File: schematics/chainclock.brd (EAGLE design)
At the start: 72.7 x 40 mm, 19 parts, among them SW1 ROTARTY_ENCODER

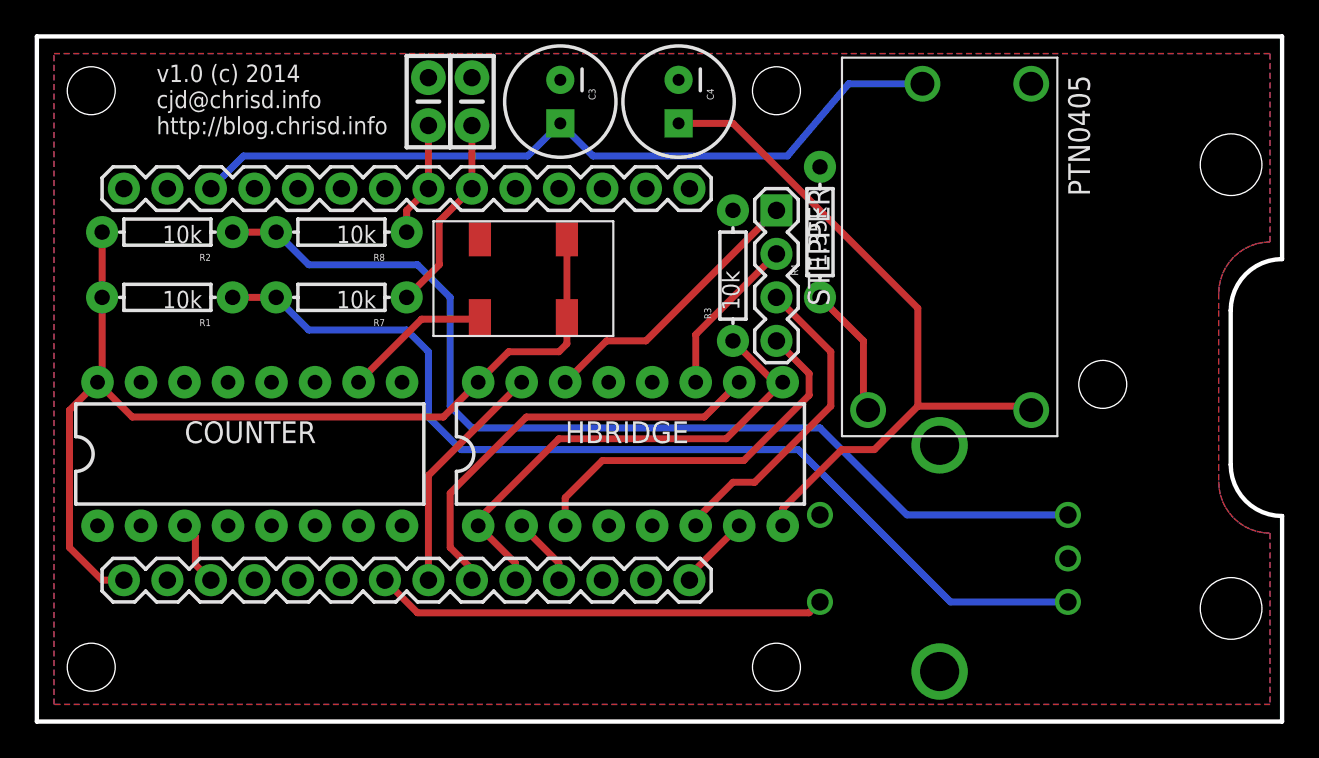
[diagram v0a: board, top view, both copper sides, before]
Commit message: New board layout
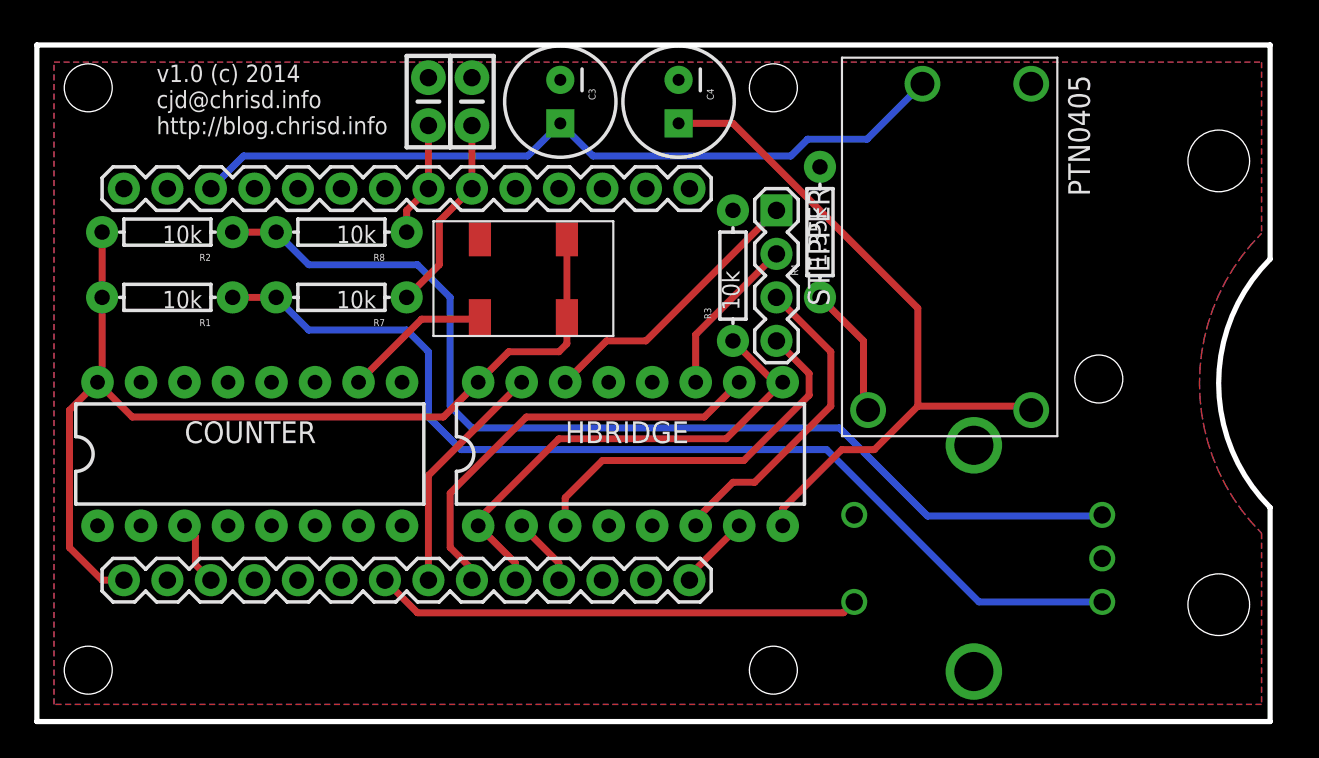
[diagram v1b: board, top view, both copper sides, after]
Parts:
- moved U$2 25.8 mm to (81.8, 19.9)
- moved SW1 2.00 mm to (54.7, 9.53)
- moved U$3 1.00 mm to (66.9, 29.8)
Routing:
- net N$5: track 59.3 -> 61.4 mm
- net N$2: track 58.4 -> 60.4 mm
- net RENBTN: track 26.5 -> 28.5 mm
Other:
- board size 72.7 x 40 mm -> 72 x 39.5 mm
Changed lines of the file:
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@@
 <setting verticaltext="up"/>
 </settings>
-<grid distance="0.025" unitdist="inch" unit="inch" style="lines" multiple="1" display="yes" altdistance="0.025" altunitdist="inch" altunit="inch"/>
+<grid distance="0.5" unitdist="mm" unit="mm" style="lines" multiple="1" display="yes" altdistance="0.025" altunitdist="inch" altunit="inch"/>
 <layers>
 <layer number="1" name="Top" color="4" fill="1" visible="yes" active="yes"/>
@@
 <board>
 <plain>
-<hole x="3.175" y="3.175" drill="2.8"/>
-<hole x="3.175" y="36.83" drill="2.8"/>
-<wire x1="0" y1="0" x2="0" y2="40" width="0.254" layer="20"/>
-<wire x1="0" y1="40" x2="72.7" y2="40" width="0.254" layer="20"/>
-<wire x1="72.7" y1="0" x2="0" y2="0" width="0.254" layer="20"/>
-<hole x="62.23" y="19.685" drill="2.8"/>
-<wire x1="72.7" y1="0" x2="72.7" y2="12" width="0.254" layer="20"/>
-<wire x1="72.7" y1="12" x2="69.7" y2="15" width="0.254" layer="20" curve="-90"/>
-<wire x1="69.7" y1="15" x2="69.7" y2="24" width="0.254" layer="20"/>
-<wire x1="69.7" y1="24" x2="72.7" y2="27" width="0.254" layer="20" curve="-90"/>
-<wire x1="72.7" y1="27" x2="72.7" y2="40" width="0.254" layer="20"/>
+<hole x="3" y="3" drill="2.8"/>
+<hole x="3" y="37" drill="2.8"/>
+<hole x="62" y="20" drill="2.8"/>
 <text x="6.985" y="34.29" size="1.016" layer="21">v1.0 (c) 2014
 cjd@chrisd.info
 http://blog.chrisd.info</text>
-<hole x="43.18" y="3.175" drill="2.8"/>
-<hole x="43.18" y="36.83" drill="2.8"/>
+<hole x="43" y="3" drill="2.8"/>
+<hole x="43" y="37" drill="2.8"/>
+<wire x1="0" y1="0" x2="0" y2="39.5" width="0.3048" layer="20"/>
+<wire x1="0" y1="39.5" x2="72" y2="39.5" width="0.3048" layer="20"/>
+<wire x1="72" y1="39.5" x2="72" y2="27" width="0.3048" layer="20"/>
+<wire x1="72" y1="27" x2="72" y2="12.5" width="0.3048" layer="20" curve="90"/>
+<wire x1="72" y1="12.5" x2="72" y2="0" width="0.3048" layer="20"/>
+<wire x1="0" y1="0" x2="72" y2="0" width="0.3048" layer="20"/>
 </plain>
 <attributes>
@@
 <element name="C4" library="SparkFun-Passives" package="CPOL-RADIAL-100UF-25V" value="" x="37.465" y="36.195" rot="R270"/>
 <element name="R4" library="SparkFun-Resistors" package="AXIAL-0.3EZ" value="1.35k" x="45.72" y="28.575" rot="R90"/>
-<element name="U$2" library="desjardins" package="NEMA14" value="" x="100.33" y="1.905" rot="R90"/>
-<element name="U$3" library="desjardins" package="LOGO" value="" x="67.945" y="29.845" rot="MR270"/>
-<element name="SW1" library="SparkFun-Electromechanical" package="ROTARY_ENC_PLAIN" value="ROTARTY_ENCODER" x="52.705" y="9.525" rot="MR180"/>
+<element name="U$2" library="desjardins" package="NEMA14" value="" x="81.83" y="19.905" rot="R90"/>
+<element name="U$3" library="desjardins" package="LOGO" value="" x="66.945" y="29.845" rot="MR270"/>
+<element name="SW1" library="SparkFun-Electromechanical" package="ROTARY_ENC_PLAIN" value="ROTARTY_ENCODER" x="54.705" y="9.525" rot="MR180"/>
 <element name="C5" library="SparkFun-Capacitors" package="CAP-PTH-SMALL-KIT" value=".01uf" x="22.86" y="36.195" rot="R90"/>
 <element name="C6" library="SparkFun-Capacitors" package="CAP-PTH-SMALL-KIT" value=".01uf" x="25.4" y="36.195" rot="R90"/>
@@
 <polygon width="0.4064" layer="16">
 <vertex x="1" y="1"/>
-<vertex x="1" y="39"/>
-<vertex x="72" y="39"/>
-<vertex x="72" y="28" curve="90"/>
-<vertex x="69" y="25"/>
-<vertex x="69" y="24"/>
-<vertex x="69" y="15"/>
-<vertex x="69" y="14" curve="90"/>
-<vertex x="72" y="11"/>
-<vertex x="72" y="1"/>
+<vertex x="1" y="38.5"/>
+<vertex x="71.5" y="38.5"/>
+<vertex x="71.5" y="28.5" curve="90"/>
+<vertex x="71.5" y="11"/>
+<vertex x="71.5" y="1"/>
 </polygon>
 <polygon width="0.4064" layer="1">
 <vertex x="1" y="1"/>
-<vertex x="1" y="39"/>
-<vertex x="72" y="39"/>
-<vertex x="72" y="28" curve="90"/>
-<vertex x="69" y="25"/>
-<vertex x="69" y="24"/>
-<vertex x="69" y="15"/>
-<vertex x="69" y="14" curve="90"/>
-<vertex x="72" y="11"/>
-<vertex x="72" y="1"/>
+<vertex x="1" y="38.5"/>
+<vertex x="71.5" y="38.5"/>
+<vertex x="71.5" y="28.5" curve="90"/>
+<vertex x="71.5" y="11"/>
+<vertex x="71.5" y="1"/>
 </polygon>
 </signal>
@@
 <wire x1="10.16" y1="31.115" x2="12.065" y2="33.02" width="0.4064" layer="16"/>
 <wire x1="12.065" y1="33.02" x2="28.655" y2="33.02" width="0.4064" layer="16"/>
-<wire x1="51.704" y1="37.236" x2="47.396" y2="37.236" width="0.4064" layer="16"/>
-<wire x1="47.396" y1="37.236" x2="43.815" y2="33.02" width="0.4064" layer="16"/>
 <wire x1="28.655" y1="33.02" x2="30.56" y2="34.925" width="0.4064" layer="16"/>
-<wire x1="43.815" y1="33.02" x2="32.465" y2="33.02" width="0.4064" layer="16"/>
+<wire x1="44.02" y1="33.02" x2="32.465" y2="33.02" width="0.4064" layer="16"/>
 <wire x1="32.465" y1="33.02" x2="30.56" y2="34.925" width="0.4064" layer="16"/>
+<wire x1="44.02" y1="33.02" x2="45" y2="34" width="0.4064" layer="16"/>
+<wire x1="45" y1="34" x2="48.468" y2="34" width="0.4064" layer="16"/>
+<wire x1="48.468" y1="34" x2="51.704" y2="37.236" width="0.4064" layer="16"/>
 </signal>
 <signal name="3V32">
@@
 <wire x1="15.875" y1="22.86" x2="21.59" y2="22.86" width="0.4064" layer="16"/>
 <wire x1="22.86" y1="17.78" x2="24.765" y2="15.875" width="0.4064" layer="16"/>
-<wire x1="24.765" y1="15.875" x2="44.45" y2="15.875" width="0.4064" layer="16"/>
-<wire x1="44.45" y1="15.875" x2="53.34" y2="6.985" width="0.4064" layer="16"/>
-<wire x1="53.34" y1="6.985" x2="60.198" y2="6.985" width="0.4064" layer="16"/>
+<wire x1="24.765" y1="15.875" x2="46.11" y2="15.875" width="0.4064" layer="16"/>
+<wire x1="55" y1="6.985" x2="62.198" y2="6.985" width="0.4064" layer="16"/>
 <wire x1="22.86" y1="17.78" x2="22.86" y2="21.59" width="0.4064" layer="16"/>
 <wire x1="22.86" y1="21.59" x2="21.59" y2="22.86" width="0.4064" layer="16"/>
+<wire x1="46.11" y1="15.875" x2="55" y2="6.985" width="0.4064" layer="16"/>
 </signal>
 <signal name="N$5">
@@
 <wire x1="24.13" y1="24.765" x2="24.13" y2="18.415" width="0.4064" layer="16"/>
 <wire x1="24.13" y1="18.415" x2="25.4" y2="17.145" width="0.4064" layer="16"/>
-<wire x1="25.4" y1="17.145" x2="45.72" y2="17.145" width="0.4064" layer="16"/>
-<wire x1="45.72" y1="17.145" x2="50.8" y2="12.065" width="0.4064" layer="16"/>
-<wire x1="50.8" y1="12.065" x2="60.198" y2="12.065" width="0.4064" layer="16"/>
+<wire x1="25.4" y1="17.145" x2="46.855" y2="17.145" width="0.4064" layer="16"/>
+<wire x1="46.855" y1="17.145" x2="52" y2="12" width="0.4064" layer="16"/>
+<wire x1="52" y1="12" x2="62.133" y2="12" width="0.4064" layer="16"/>
+<wire x1="62.133" y1="12" x2="62.198" y2="12.065" width="0.4064" layer="16"/>
 </signal>
 <signal name="RENBTN">
 <contactref element="SW1" pad="SW+"/>
 <contactref element="ARDUNOFIO" pad="7"/>
-<wire x1="45.085" y1="6.35" x2="22.225" y2="6.35" width="0.4064" layer="1"/>
+<wire x1="47.085" y1="6.35" x2="22.225" y2="6.35" width="0.4064" layer="1"/>
 <wire x1="22.225" y1="6.35" x2="20.32" y2="8.255" width="0.4064" layer="1"/>
-<wire x1="45.085" y1="6.35" x2="45.72" y2="6.985" width="0.4064" layer="1"/>
+<wire x1="47.085" y1="6.35" x2="47.72" y2="6.985" width="0.4064" layer="1"/>
 </signal>
 <signal name="RENCB">
